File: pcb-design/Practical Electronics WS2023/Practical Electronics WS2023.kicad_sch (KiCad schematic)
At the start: 30 parts, among them J1 PWR Jack, J2 MIDI Input, J3 MIDI Thru out, J4 Conn_01x03, J5 ISP, Q1 Q_NMOS_DGS, SW1 SW_SPDT, SW2 SW_SPDT, SW4 SW_SPDT, U1 6N138, U1 ATmega328P-P, U2 ADP2303ARDZ-5.0, U3 74HCT04, Y1 Crystal

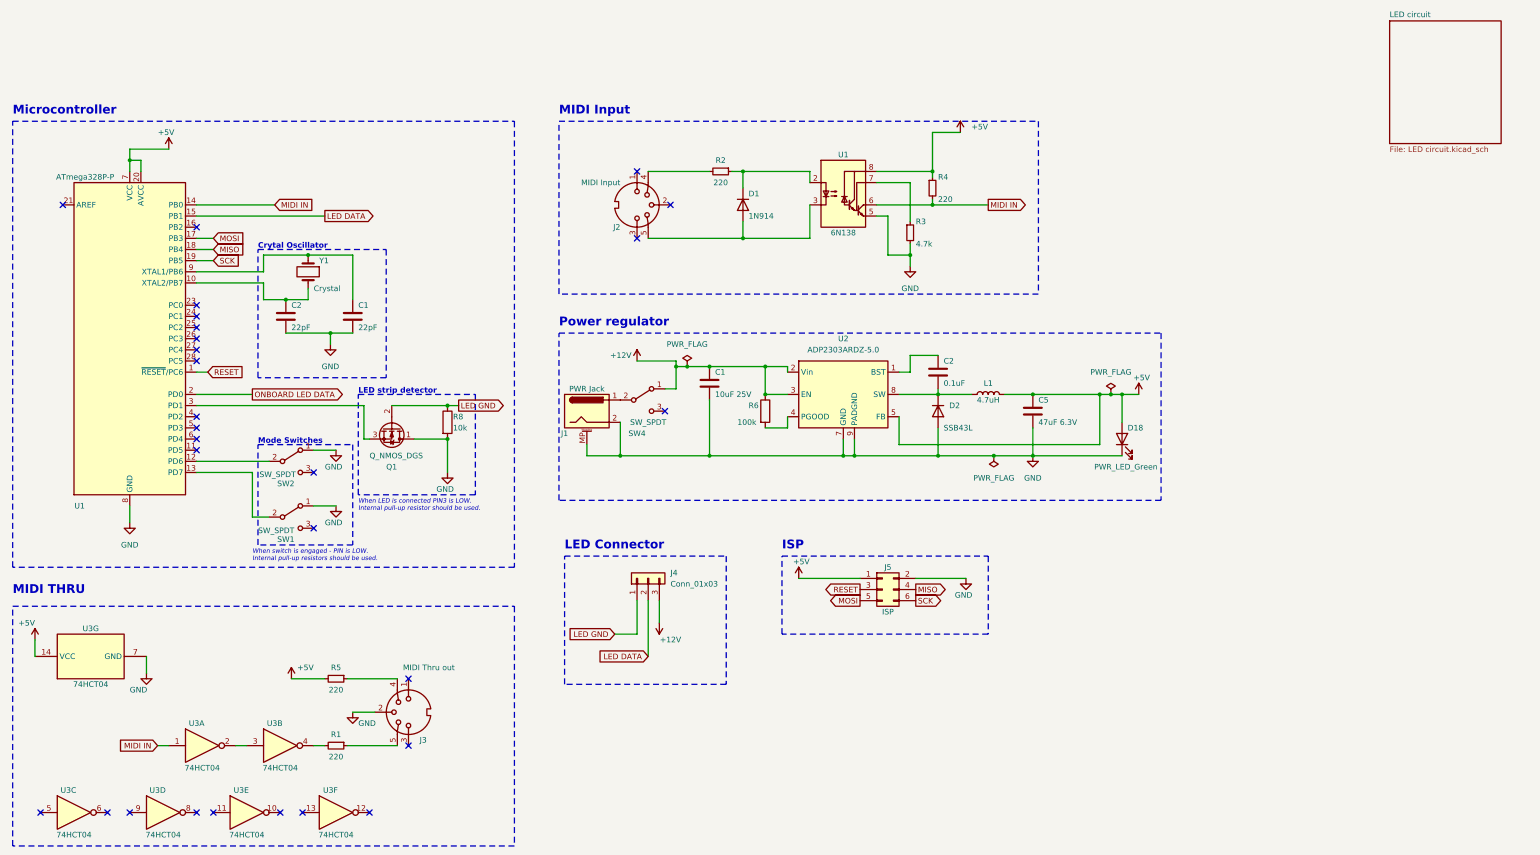
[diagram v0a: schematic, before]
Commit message: Update schematic
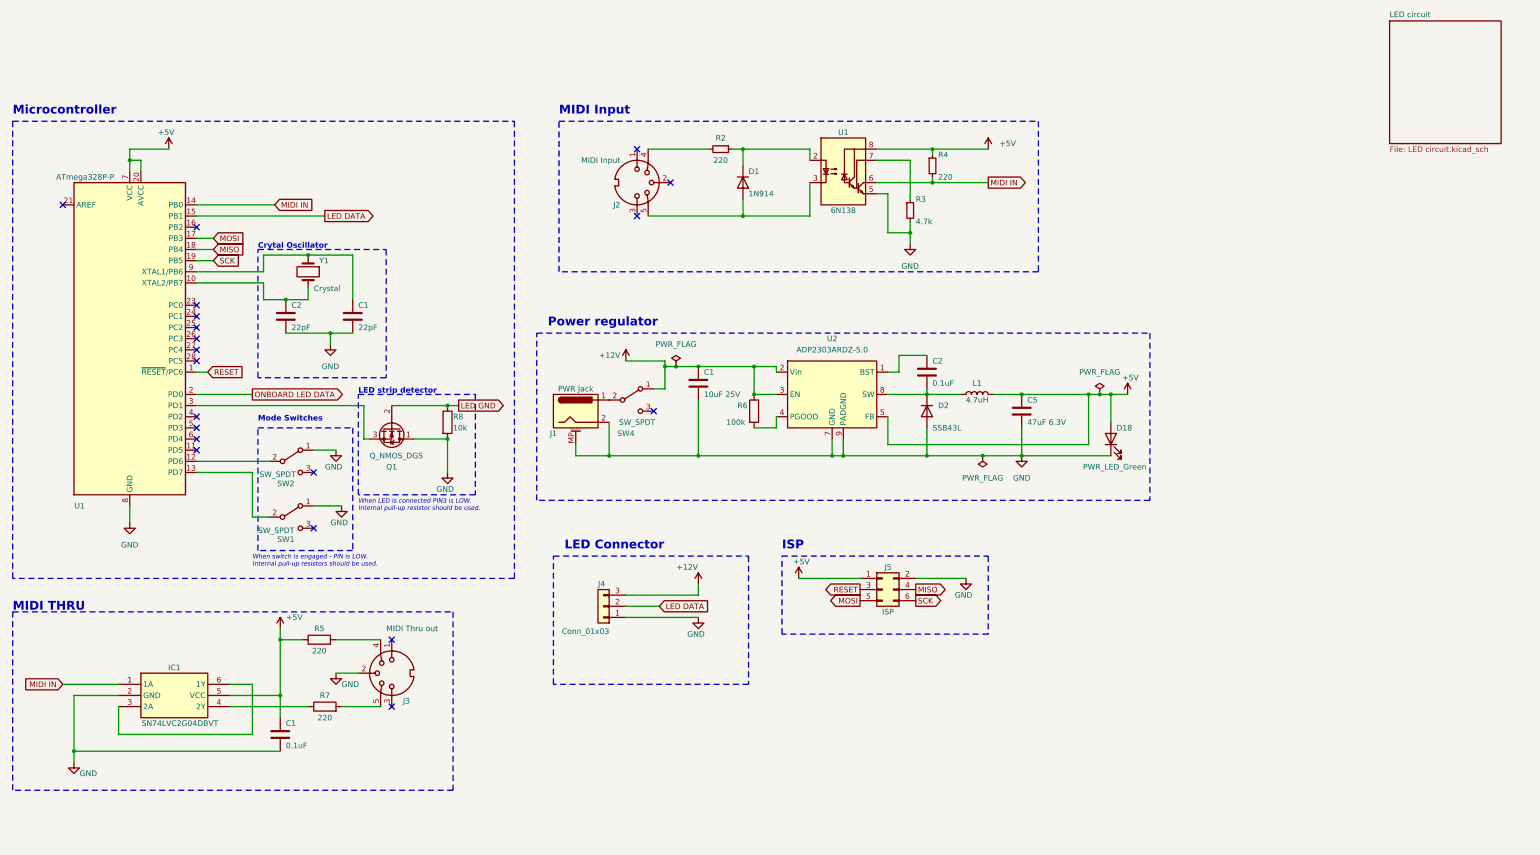
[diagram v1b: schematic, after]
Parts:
- removed R1, R5: 220, symbol Device:R_Small
- removed U3: 74HCT04, symbol 74xx:74HCT04
- added C1: 0.1uF, symbol Device:C
- added IC1: SN74LVC2G04DBVT, SOT95P280X145-6N, symbol SN74LVC2G04DBVT:SN74LVC2G04DBVT
- added R5, R7: 220, symbol Device:R
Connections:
- net +5V: now also C1.2, IC1.5 (VCC), R5.1
- net GND: now also J4.1 (Pin_1), C1.1, IC1.2 (GND)
- net LED GND: no longer J4.1 (Pin_1)
- net MIDI IN: now also IC1.1 (1A)
- net at J3.5: now also R7.2
- net at J3.4: now also R5.2
- new net: IC1.3 (2A), IC1.6 (1Y)
- new net: IC1.4 (2Y), R7.1
- no-connect marks 28 -> 20
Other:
- moved on the sheet: C1, C2, C5, D1, D18, D2, J1, J2, J3, J4, L1, R2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
